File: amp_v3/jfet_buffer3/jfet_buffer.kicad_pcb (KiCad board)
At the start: 2 copper layers, 74.9 x 28.6 mm, 24 parts, among them J1 SIG_OUT_L1, J2 SIG_OUT_L1, J3 SIG_OUT_L1, J4 SIG_OUT_L2, Q1 2N5457, Q2 2N5457 DSG

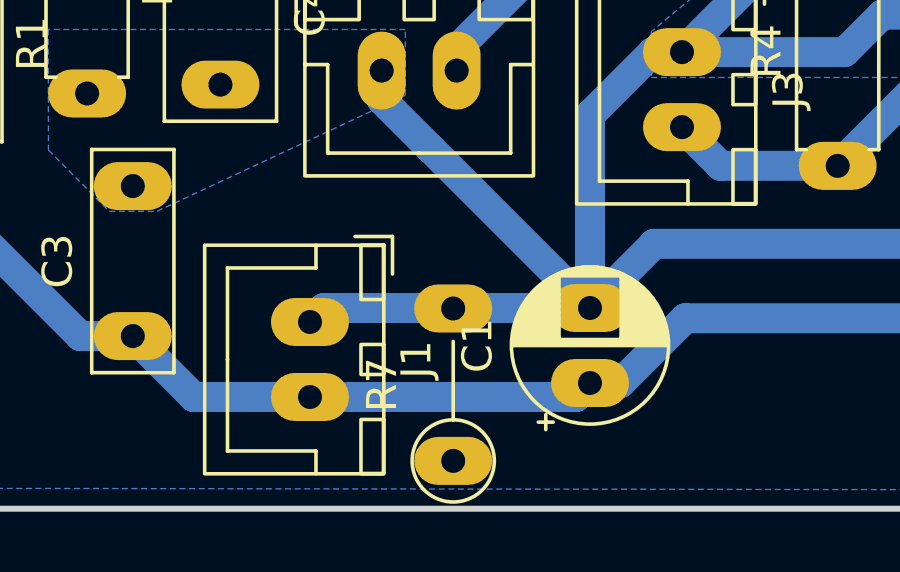
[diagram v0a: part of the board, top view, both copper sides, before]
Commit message: updates
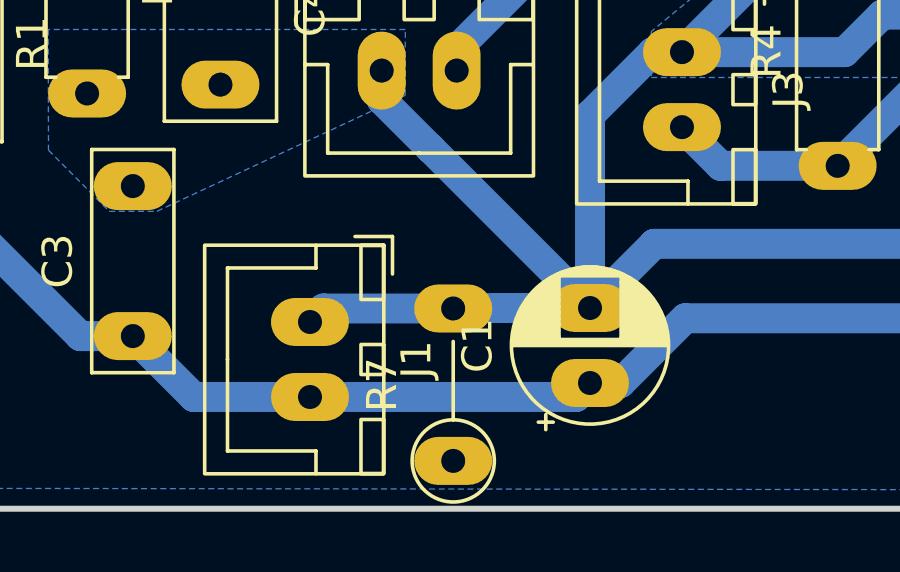
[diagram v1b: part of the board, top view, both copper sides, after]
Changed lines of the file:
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@@
-	)
-	(segment
-		(start 54.517 68.203)
-		(end 54.983 67.737)
-		(width 1)
-		(layer "B.Cu")
-		(net "GND_IN_L")
 	)
 	(segment
@@
 		(start 65.947152 59.208)
 		(end 63.852 61.303152)
+		(width 1)
+		(layer "B.Cu")
+		(net "GND_IN_L")
+	)
+	(segment
+		(start 59.292 67.753)
+		(end 54.967 67.753)
 		(width 1)
 		(layer "B.Cu")
@@
 	)
 	(segment
-		(start 54.983 67.737)
-		(end 63.852 67.737)
-		(width 1)
-		(layer "B.Cu")
-		(net "GND_IN_L")
-	)
-	(segment
 		(start 63.852 67.733)
 		(end 58.542 62.423)
@@
 	)
 	(segment
+		(start 63.852 67.737)
+		(end 59.308 67.737)
+		(width 1)
+		(layer "B.Cu")
+		(net "GND_IN_L")
+	)
+	(segment
 		(start 66.917 59.208)
 		(end 65.947152 59.208)
+		(width 1)
+		(layer "B.Cu")
+		(net "GND_IN_L")
+	)
+	(segment
+		(start 54.967 67.753)
+		(end 54.517 68.203)
 		(width 1)
 		(layer "B.Cu")
@@
 		(width 1)
 		(layer "B.Cu")
+		(net "GND_IN_L")
+	)
+	(segment
+		(start 59.308 67.737)
+		(end 59.292 67.753)
+		(width 1)
+		(layer "B.Cu")
